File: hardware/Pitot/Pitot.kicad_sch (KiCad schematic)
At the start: 32 parts, among them J1 53307-2471, J2 Conn_01x05, J3 Conn_01x04, J4 Conn_01x08, J5 Conn_01x05, J6 Conn_01x04, J7 Conn_01x04, J8 Conn_01x02

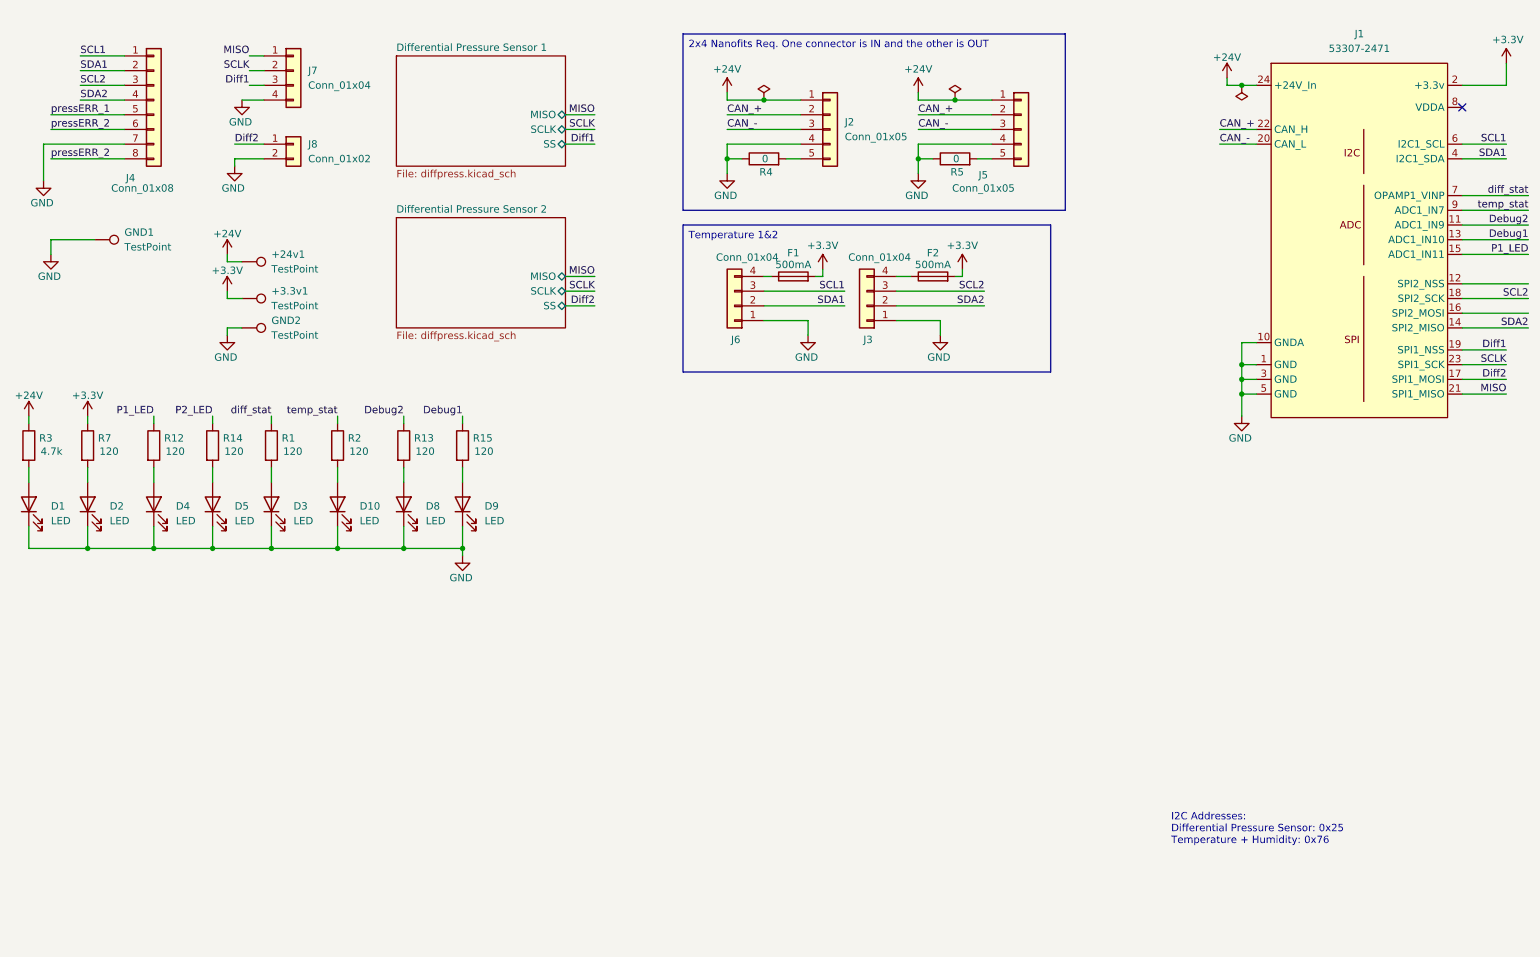
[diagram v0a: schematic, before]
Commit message: ready to review
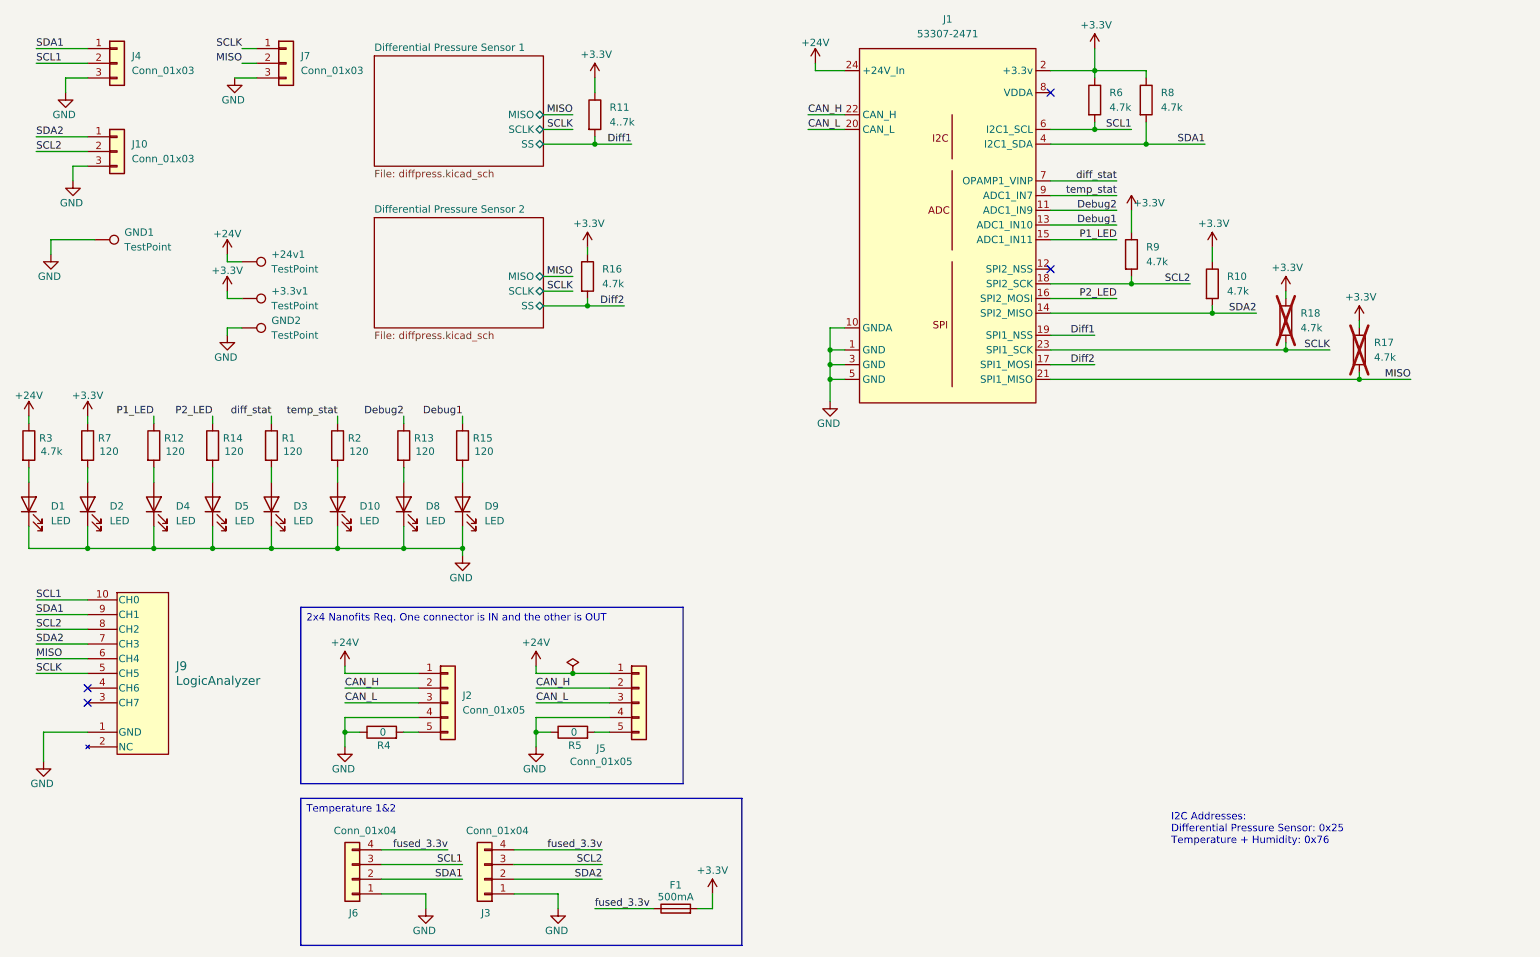
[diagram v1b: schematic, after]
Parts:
- removed F2: 500mA, Fuse:Fuse_0603_1608Metric_Pad1.05x0.95mm_HandSolder, symbol Device:Fuse
- removed J4: Conn_01x08, Connector_PinHeader_2.54mm:PinHeader_2x04_P2.54mm_Vertical, symbol Connector_Generic:Conn_01x08
- removed J7: Conn_01x04, Connector_PinHeader_2.54mm:PinHeader_1x04_P2.54mm_Vertical, symbol Connector_Generic:Conn_01x04
- removed J8: Conn_01x02, Connector_PinHeader_2.54mm:PinHeader_1x02_P2.54mm_Vertical, symbol Connector_Generic:Conn_01x02
- added J10, J4, J7: Conn_01x03, Connector_PinHeader_2.54mm:PinHeader_1x03_P2.54mm_Vertical, symbol Connector_Generic:Conn_01x03
- added J9: LogicAnalyzer, UTSVT_Connectors:CONN_SFH11-xxxC-D05-ST-XX_SUL, symbol utsvt_connectors:LogicAnalyzer
- added R10, R16, R17, R18, R6, R8, R9: 4.7k, Resistor_SMD:R_0603_1608Metric_Pad0.98x0.95mm_HandSolder, symbol Device:R
- added R11: 4..7k, Resistor_SMD:R_0603_1608Metric_Pad0.98x0.95mm_HandSolder, symbol Device:R
- +24v1, +3.3v1, GND1, GND2: footprint TestPoint:TestPoint_Pad_1.0x1.0mm -> TestPoint:TestPoint_THTPad_2.0x2.0mm_Drill1.0mm
- J2, J5: P/N (none) -> 1053131105
- J3, J6: P/N (none) -> 1053131104
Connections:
- net +3.3V: now also R10.1, R11.1, R16.1, R17.1, R18.1, R6.1, R8.1, R9.1
- net Diff1: now also R11.2
- net Diff2: now also R16.2
- net GND: now also J10.3 (Pin_3), J4.3 (Pin_3), J7.3 (Pin_3), J9.1 (GND)
- net MISO: now also J7.2 (Pin_2), J9.6 (CH4), R17.2
- net P2_LED: now also J1.16 (SPI2_MOSI)
- net SCL1: now also J4.2 (Pin_2), J9.10 (CH0), R6.2
- net SCL2: now also J10.2 (Pin_2), J9.8 (CH2), R9.2
- net SCLK: now also J7.1 (Pin_1), J9.5 (CH5), R18.2
- net SDA1: now also J4.1 (Pin_1), J9.9 (CH1), R8.2
- net SDA2: now also J10.1 (Pin_1), J9.7 (CH3), R10.2
- net fused_3.3v: now reaches F1.1, J6.4 (Pin_4)
- net fused_3.3v: now also J3.4 (Pin_4)
- net CAN_+ renamed CAN_H
- net CAN_- renamed CAN_L
- no-connect marks 1 -> 4
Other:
- moved on the sheet: J1, J2, J3, J5, J6, R4, R5
